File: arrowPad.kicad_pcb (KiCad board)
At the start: 2 copper layers, 69.8 x 61.2 mm, 28 parts, among them K1 KEYSW, K2 KEYSW, K3 KEYSW, K4 KEYSW, K5 KEYSW, K6 KEYSW, K7 KEYSW, K8 KEYSW, K9 KEYSW, SW1 SW_DIP_x01, U1 ProMicro, U2 NRF24L01_Breakout

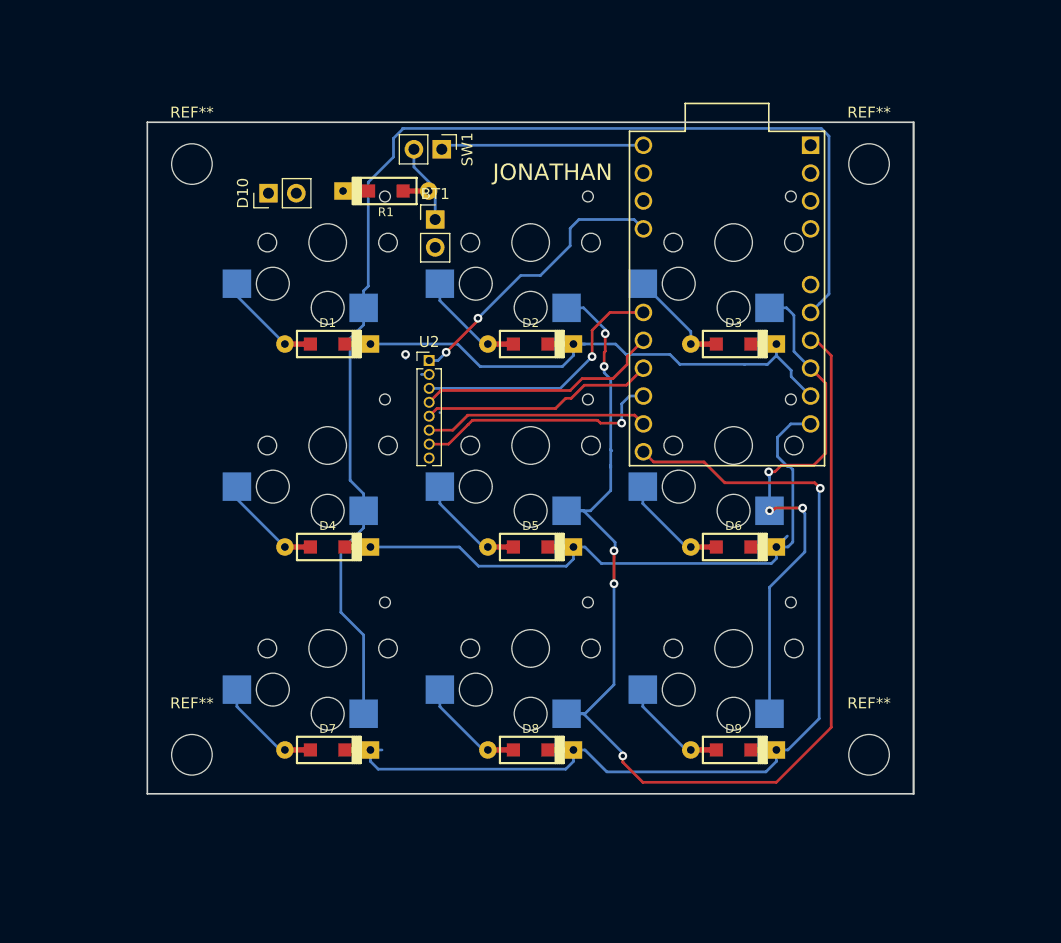
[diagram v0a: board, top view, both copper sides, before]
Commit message: final v1
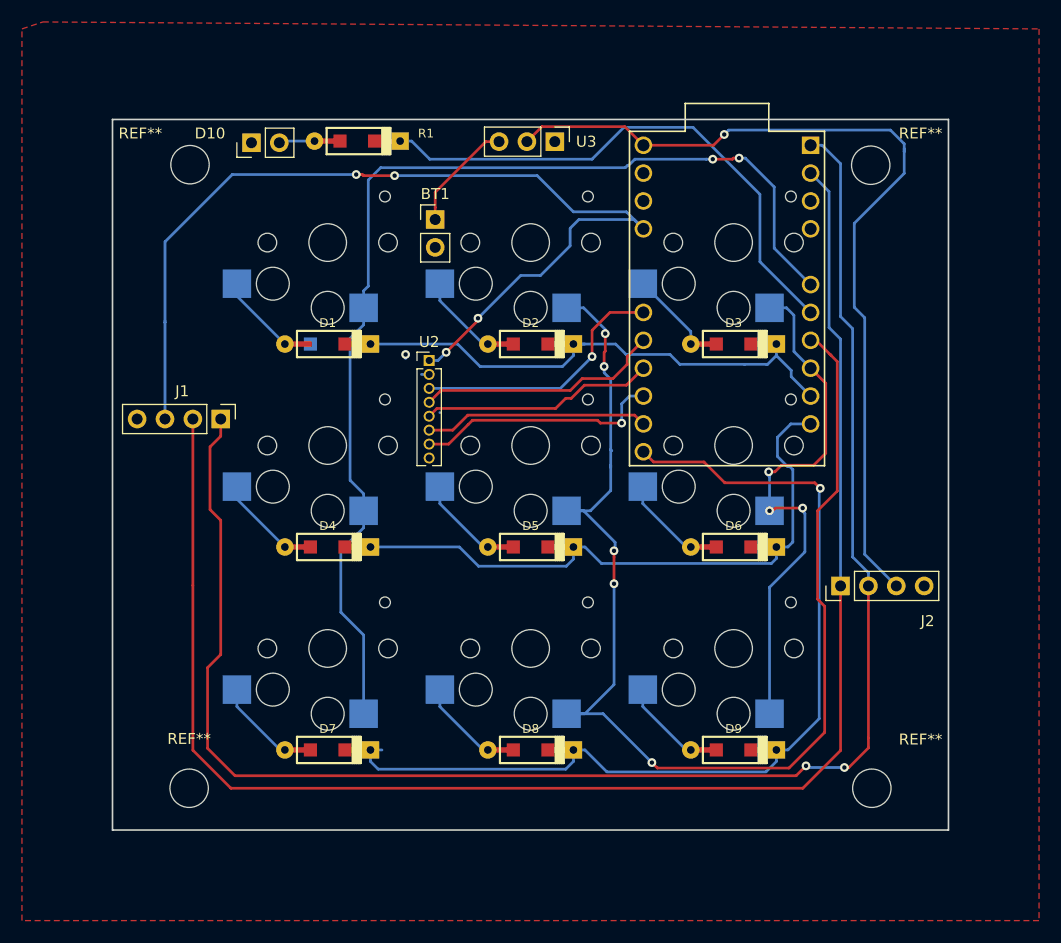
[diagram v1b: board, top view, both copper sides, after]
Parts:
- removed the REF** at (101.3, 139.2)
- removed the REF** at (39.6, 85.3)
- removed the REF** at (39.6, 139.2)
- removed the REF** at (101.3, 85.3)
- removed SW1: SW_DIP_x01, Connector_PinHeader_2.54mm:PinHeader_1x02_P2.54mm_Vertical
- added J1: AudioJack3_Ground, Connector_PinHeader_2.54mm:PinHeader_1x04_P2.54mm_Vertical, F.Cu at (42.2, 108.6)
- added J2: AudioJack3_Ground, Connector_PinHeader_2.54mm:PinHeader_1x04_P2.54mm_Vertical, F.Cu at (98.8, 123.8)
- added REF**: MountingHole_3.5mm, MountingHole:MountingHole_3.5mm, F.Cu at (101.5, 85.5)
- added REF**: MountingHole_3.5mm, MountingHole:MountingHole_3.5mm, F.Cu at (39.5, 85.4)
- added REF**: MountingHole_3.5mm, MountingHole:MountingHole_3.5mm, F.Cu at (101.6, 142.2)
- added REF**: MountingHole_3.5mm, MountingHole:MountingHole_3.5mm, F.Cu at (39.4, 142.2)
- added U3: ADG417BN, Connector_PinHeader_2.54mm:PinHeader_1x03_P2.54mm_Vertical, F.Cu at (72.7, 83.3)
- moved R1 5.24 mm to (54.7, 83.2), turned to 180 degrees
- moved D10 4.85 mm to (45.0, 83.4)
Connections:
- R1 pad 1: Net-(D10-Pad2) -> Net-(R1-Pad1)
- R1 pad 2: Net-(R1-Pad2) -> Net-(D10-Pad2)
- U1 pad 6: Net-(R1-Pad2) -> /Col1
- U1 pad 7: /Col1 -> Net-(R1-Pad1)
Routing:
- net Net-(J1-Pad1): track 0.00 -> 151.5 mm, vias 0 -> 2
- net Net-(J1-Pad2): track 0.00 -> 145.8 mm
- net Net-(J1-Pad3): track 26.3 -> 90.8 mm, vias 2 -> 4
- net /RAW1: track 18.5 -> 81.0 mm, vias 0 -> 1
- net Net-(R1-Pad1): track 0.00 -> 49.9 mm
- net /Col1: track 113.5 -> 100.8 mm, vias 0 -> 2
- net Net-(D10-Pad2): track 0.00 -> 3.41 mm
- net Net-(BT1-Pad1): track 7.20 -> 10.2 mm
- net /Row2: track 57.8 -> 56.4 mm
- net /Col2: track 114.3 -> 115.3 mm
- added copper zone on F.Cu, net /GND1
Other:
- board size 69.8 x 61.2 mm -> 76.2 x 64.8 mm
- board text removed: "JONATHAN"
